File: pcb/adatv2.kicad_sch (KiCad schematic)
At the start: 0 parts

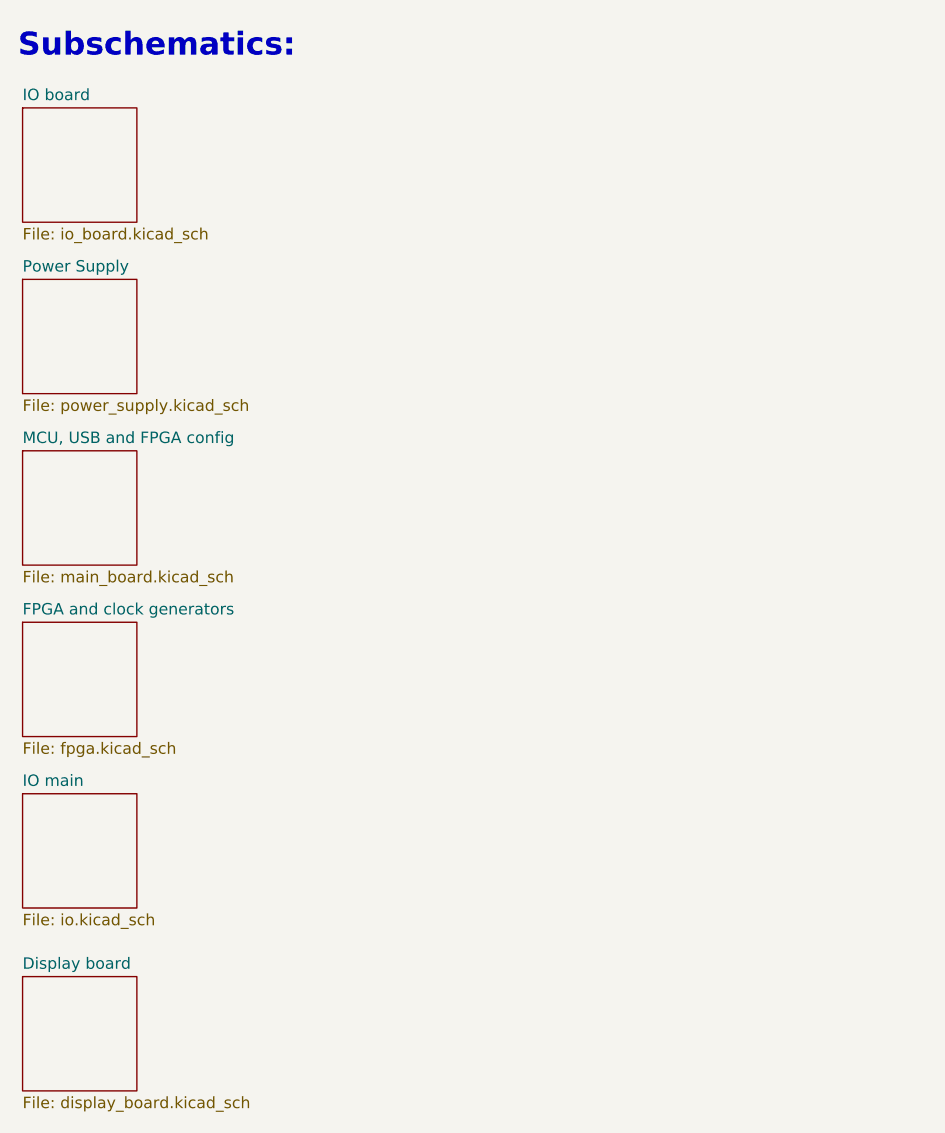
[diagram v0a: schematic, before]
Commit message: Further schematic capture
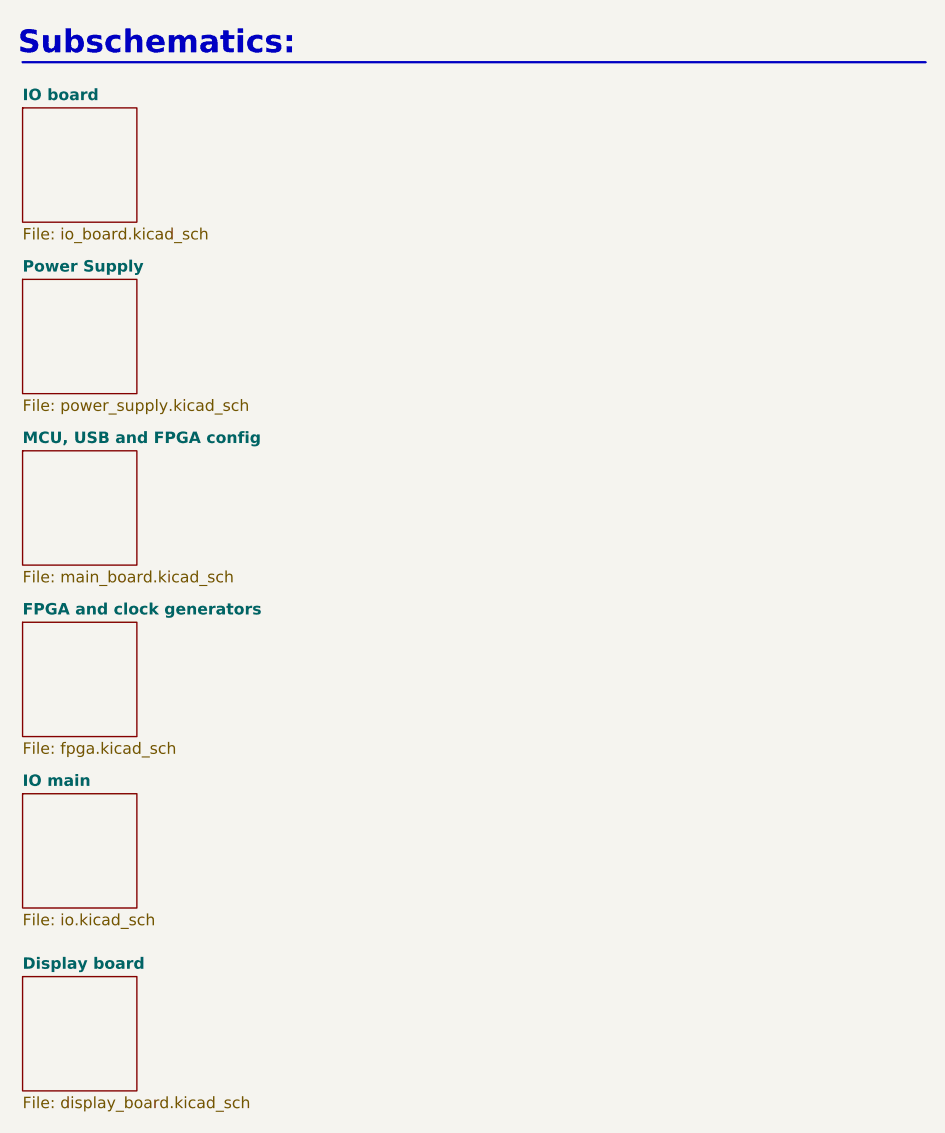
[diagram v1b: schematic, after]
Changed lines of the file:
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@@
 	(text "Subschematics:"
 		(exclude_from_sim no)
-		(at 177.292 28.702 0)
+		(at 177.292 28.448 0)
 		(effects
 			(font
@@
 		)
 	)
+	(polyline
+		(pts
+			(xy 177.8 30.48) (xy 278.13 30.48)
+		)
+		(stroke
+			(width 0.254)
+			(type solid)
+		)
+	)
 	(sheet
 		(at 177.8 35.56)
@@
 				(font
 					(size 1.27 1.27)
+					(thickness 0.254)
+					(bold yes)
 				)
 				(justify left bottom)
@@
 				(font
 					(size 1.27 1.27)
+					(thickness 0.254)
+					(bold yes)
 				)
 				(justify left bottom)
@@
 				(font
 					(size 1.27 1.27)
+					(thickness 0.254)
+					(bold yes)
 				)
 				(justify left bottom)
@@
 				(font
 					(size 1.27 1.27)
+					(thickness 0.254)
+					(bold yes)
 				)
 				(justify left bottom)
@@
 				(font
 					(size 1.27 1.27)
+					(thickness 0.254)
+					(bold yes)
 				)
 				(justify left bottom)
@@
 				(font
 					(size 1.27 1.27)
-				)
-				(justify left bottom)
+					(thickness 0.254)
+					(bold yes)
+				)
+				(justify left bottom)
